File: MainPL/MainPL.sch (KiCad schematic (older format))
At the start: 37 parts, among them J1 Conn_01x06_Female, J10 Conn_01x06_Female, J11 Conn_01x06_Female, J12 Conn_01x06_Female, J13 Conn_01x06_Female, J14 Conn_01x06_Female, J15 Conn_01x01_Male, J16 Conn_01x04_Male, J2 USB_B, J3 Conn_01x06_Female, J4 Conn_01x06_Female, J5 Conn_01x06_Female, J6 Conn_01x06_Female, J7 Conn_01x09_Male, J8 Conn_01x06_Female, J9 Conn_01x06_Female, SW1 SW_Push_Dual, U1 74LS32, U2 ATmega328P-PU, U3 MCP23017_SP, U5 MCP23017_SP, U6 74LS373, U7 MCP23017_SP, U8 MC74HC589A, U9 74LVC2G04, Y1 Crystal_GND2

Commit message: Verbesserung fehlt
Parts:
- C2, C4: footprint Capacitor_SMD:C_1206_3216Metric_Pad1.42x1.75mm_HandSolder -> Capacitor_SMD:C_0805_2012Metric_Pad1.15x1.40mm_HandSolder
- D1: footprint Diode_THT:D_5W_P12.70mm_Horizontal -> Diode_THT:D_5W_P10.16mm_Horizontal
- R5, R7: footprint Resistor_SMD:R_1206_3216Metric_Pad1.42x1.75mm_HandSolder -> Resistor_SMD:R_0805_2012Metric_Pad1.15x1.40mm_HandSolder
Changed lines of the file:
@@
 EESchema Schematic File Version 4
+LIBS:MainPL-cache
 EELAYER 30 0
 EELAYER END
@@
 F 0 "C2" H 6115 8496 50  0000 L CNN
 F 1 "100n" H 6115 8405 50  0000 L CNN
-F 2 "Capacitor_SMD:C_1206_3216Metric_Pad1.42x1.75mm_HandSolder" H 6038 8300 50  0001 C CNN
+F 2 "Capacitor_SMD:C_0805_2012Metric_Pad1.15x1.40mm_HandSolder" H 6038 8300 50  0001 C CNN
 F 3 "~" H 6000 8450 50  0001 C CNN
 	1    6000 8450
@@
 F 0 "R5" H 6275 6800 50  0000 L CNN
 F 1 "1M" H 6400 6775 50  0000 L CNN
-F 2 "Resistor_SMD:R_1206_3216Metric_Pad1.42x1.75mm_HandSolder" V 6355 6775 50  0001 C CNN
+F 2 "Resistor_SMD:R_0805_2012Metric_Pad1.15x1.40mm_HandSolder" V 6355 6775 50  0001 C CNN
 F 3 "~" H 6425 6775 50  0001 C CNN
 	1    6425 6775
@@
 F 0 "C4" H 7440 8721 50  0000 L CNN
 F 1 "100n" H 7440 8630 50  0000 L CNN
-F 2 "Capacitor_SMD:C_1206_3216Metric_Pad1.42x1.75mm_HandSolder" H 7363 8525 50  0001 C CNN
+F 2 "Capacitor_SMD:C_0805_2012Metric_Pad1.15x1.40mm_HandSolder" H 7363 8525 50  0001 C CNN
 F 3 "~" H 7325 8675 50  0001 C CNN
 	1    7325 8675
@@
 F 0 "D1" V 7596 6146 50  0000 R CNN
 F 1 "D" V 7505 6146 50  0000 R CNN
-F 2 "Diode_THT:D_5W_P12.70mm_Horizontal" H 7550 6225 50  0001 C CNN
+F 2 "Diode_THT:D_5W_P10.16mm_Horizontal" H 7550 6225 50  0001 C CNN
 F 3 "~" H 7550 6225 50  0001 C CNN
 	1    7550 6225
@@
 F 0 "R7" V 7343 6000 50  0000 C CNN
 F 1 "10k" V 7434 6000 50  0000 C CNN
-F 2 "Resistor_SMD:R_1206_3216Metric_Pad1.42x1.75mm_HandSolder" V 7480 6000 50  0001 C CNN
+F 2 "Resistor_SMD:R_0805_2012Metric_Pad1.15x1.40mm_HandSolder" V 7480 6000 50  0001 C CNN
 F 3 "~" H 7550 6000 50  0001 C CNN
 	1    7550 6000

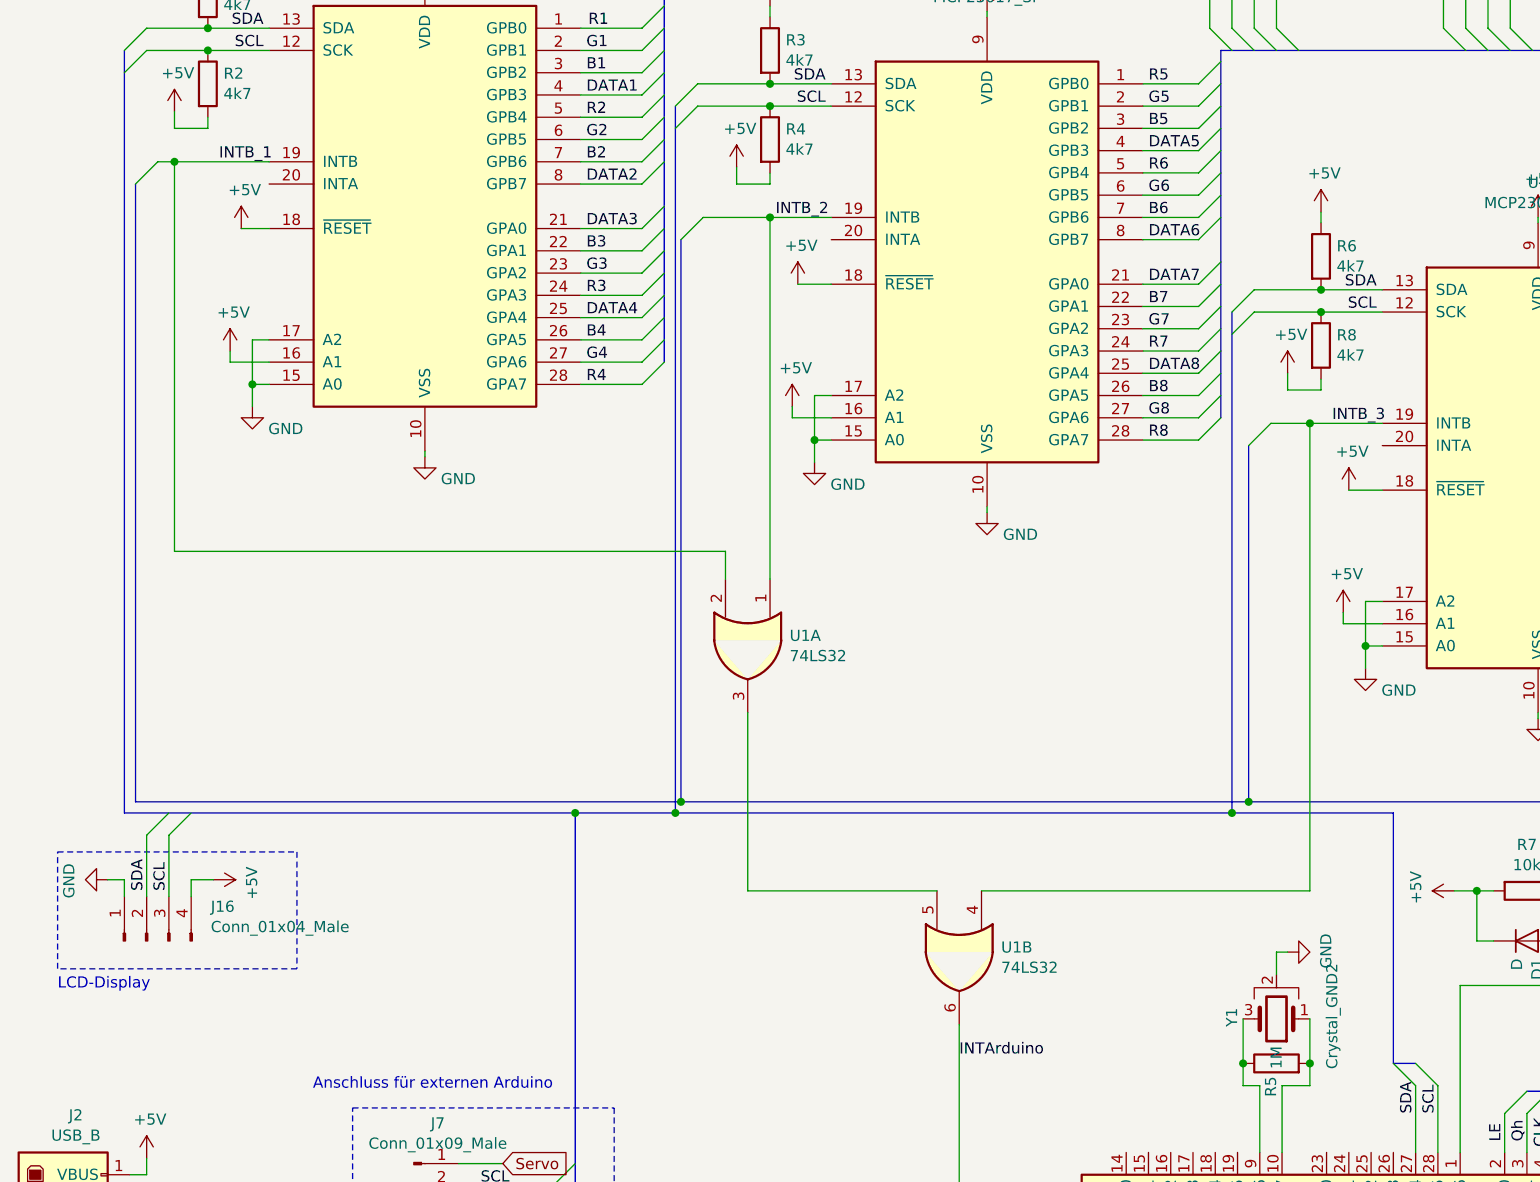
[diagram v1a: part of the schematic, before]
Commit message: File gefixed
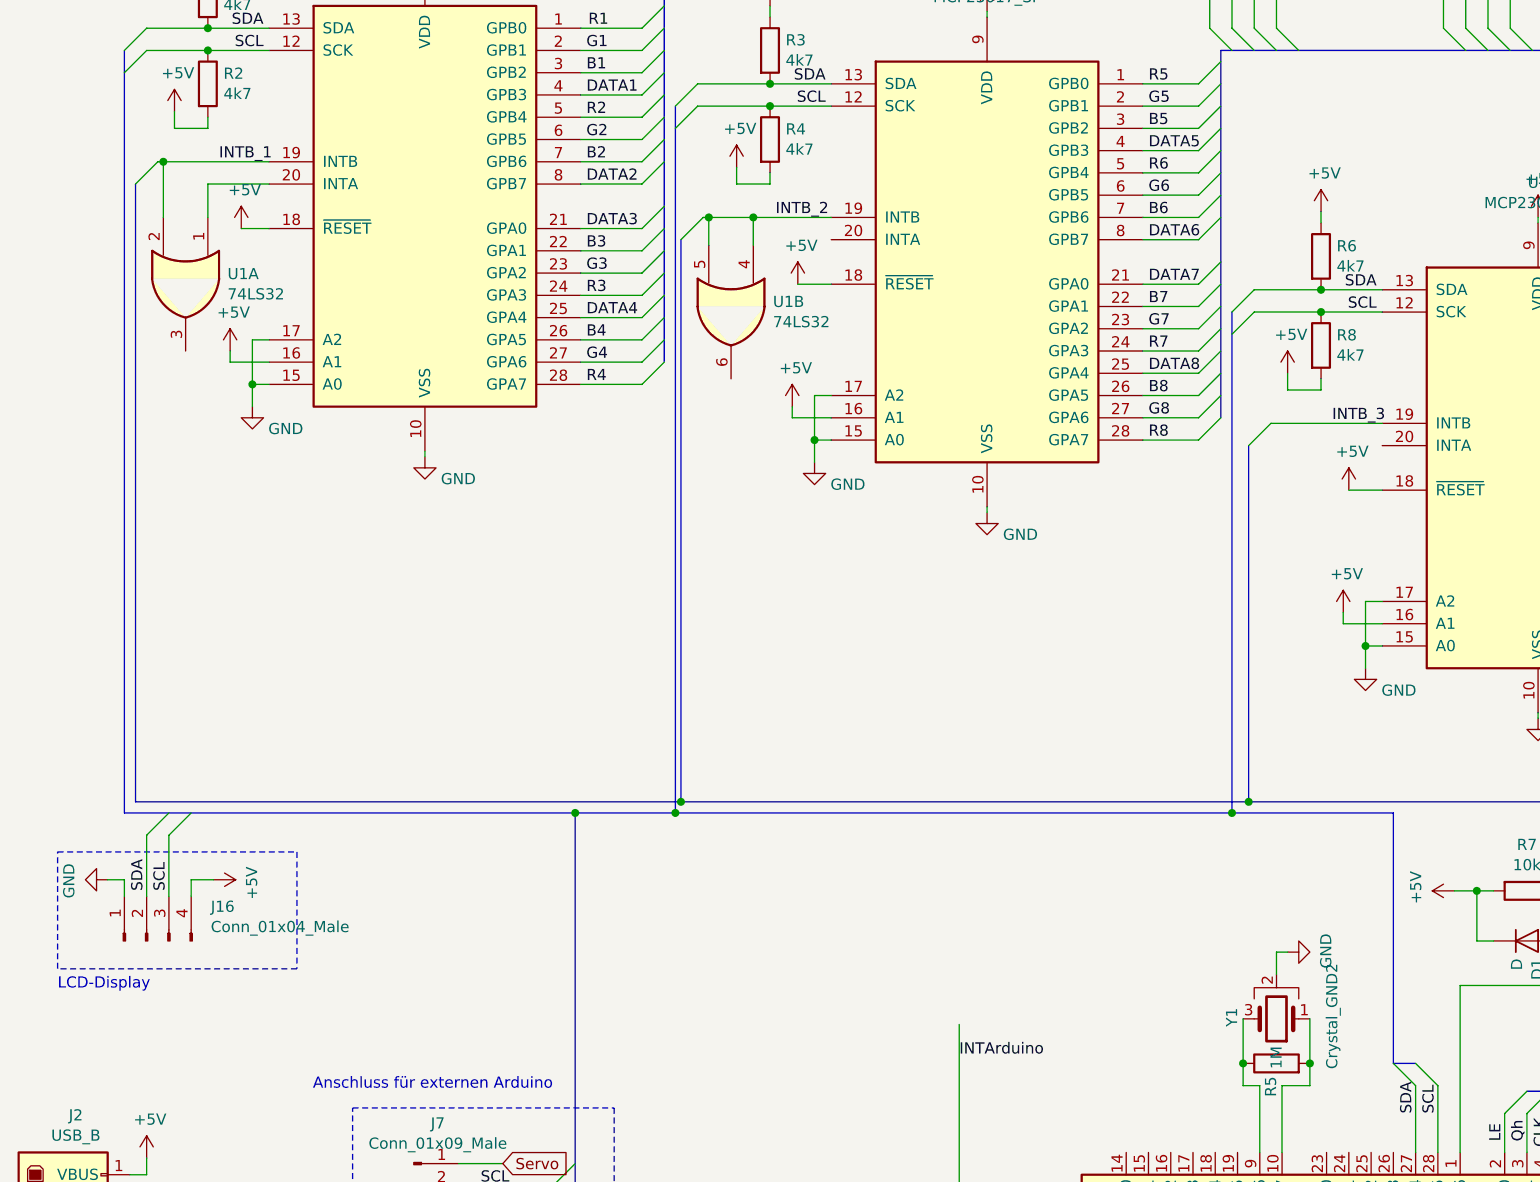
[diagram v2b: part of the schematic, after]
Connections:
- net INTArduino: no longer U1.6
- net INTB_2: now also U1.4, U1.5; no longer U1.1
- net INTB_3: no longer U1.4
- net at U1.3: no longer U1.5
- net at U3.20 (INTA): now also U1.1
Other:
- moved on the sheet: U1A, U1B
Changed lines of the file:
@@
 EESchema Schematic File Version 4
-LIBS:MainPL-cache
 EELAYER 30 0
 EELAYER END
@@
 Wire Wire Line
 	8725 6150 8725 6250
-Wire Wire Line
-	1400 2725 1475 2725
-Wire Wire Line
-	3850 2975 4150 2975
-Wire Wire Line
-	6400 3900 6575 3900
 $Comp
 L 74xx:74LS32 U1
 U 1 1 5E03B617
-P 4050 4900
-F 0 "U1" V 4004 5088 50  0000 L CNN
-F 1 "74LS32" V 4095 5088 50  0000 L CNN
-F 2 "Package_DIP:DIP-14_W7.62mm_Socket_LongPads" H 4050 4900 50  0001 C CNN
-F 3 "http://www.ti.com/lit/gpn/sn74LS32" H 4050 4900 50  0001 C CNN
-	1    4050 4900
+P 1525 3275
+F 0 "U1" V 1479 3463 50  0000 L CNN
+F 1 "74LS32" V 1570 3463 50  0000 L CNN
+F 2 "Package_DIP:DIP-14_W7.62mm_Socket_LongPads" H 1525 3275 50  0001 C CNN
+F 3 "http://www.ti.com/lit/gpn/sn74LS32" H 1525 3275 50  0001 C CNN
+	1    1525 3275
 	0    1    1    0
 $EndComp
-Wire Wire Line
-	1475 2725 1475 4475
-Wire Wire Line
-	1475 4475 3950 4475
-Wire Wire Line
-	3950 4475 3950 4600
-Connection ~ 1475 2725
-Wire Wire Line
-	1475 2725 1900 2725
-Wire Wire Line
-	4150 4600 4150 2975
-Connection ~ 4150 2975
-Wire Wire Line
-	4150 2975 4425 2975
-Connection ~ 6575 3900
-Wire Wire Line
-	6575 3900 6900 3900
-Wire Wire Line
-	4050 5200 4050 6000
-Wire Wire Line
-	4050 6000 4900 6000
-Wire Wire Line
-	5100 6000 6575 6000
-Wire Wire Line
-	6575 3900 6575 6000
 Wire Bus Line
 	1300 2825 1300 5600
@@
 L 74xx:74LS32 U1
 U 2 1 5E02EBD5
-P 5000 6300
-F 0 "U1" V 4954 6488 50  0000 L CNN
-F 1 "74LS32" V 5045 6488 50  0000 L CNN
-F 2 "Package_DIP:DIP-14_W7.62mm_Socket_LongPads" H 5000 6300 50  0001 C CNN
-F 3 "http://www.ti.com/lit/gpn/sn74LS32" H 5000 6300 50  0001 C CNN
-	2    5000 6300
+P 3975 3400
+F 0 "U1" V 3929 3588 50  0000 L CNN
+F 1 "74LS32" V 4020 3588 50  0000 L CNN
+F 2 "Package_DIP:DIP-14_W7.62mm_Socket_LongPads" H 3975 3400 50  0001 C CNN
+F 3 "http://www.ti.com/lit/gpn/sn74LS32" H 3975 3400 50  0001 C CNN
+	2    3975 3400
 	0    1    1    0
 $EndComp
@@
 Text Notes 950  6450 0    50   ~ 0
 LCD-Display
+Wire Wire Line
+	1400 2725 1425 2725
+Wire Wire Line
+	1425 2975 1425 2725
+Connection ~ 1425 2725
+Wire Wire Line
+	1425 2725 1900 2725
+Wire Wire Line
+	1625 2975 1625 2825
+Wire Wire Line
+	1625 2825 1900 2825
+Wire Wire Line
+	3850 2975 3875 2975
+Wire Wire Line
+	3875 3100 3875 2975
+Connection ~ 3875 2975
+Wire Wire Line
+	3875 2975 4075 2975
+Wire Wire Line
+	4075 3100 4075 2975
 Wire Bus Line
 	1250 2225 1250 5650
@@
 Wire Bus Line
 	3675 1250 7450 1250
+Connection ~ 4075 2975
+Wire Wire Line
+	4075 2975 4425 2975
+Wire Wire Line
+	6400 3900 6900 3900
 $EndSCHEMATC
